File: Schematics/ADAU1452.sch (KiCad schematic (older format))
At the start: 97 parts, among them CN201 COAX, P201 CONN_2x1, P202 CONN_6X2, P203 CONN_6x1, SW201 SWITCH, U201 ADAU1452WBCPZ, U202 ADM13307-5ARZ, U203 25AA1024, X201 24M576

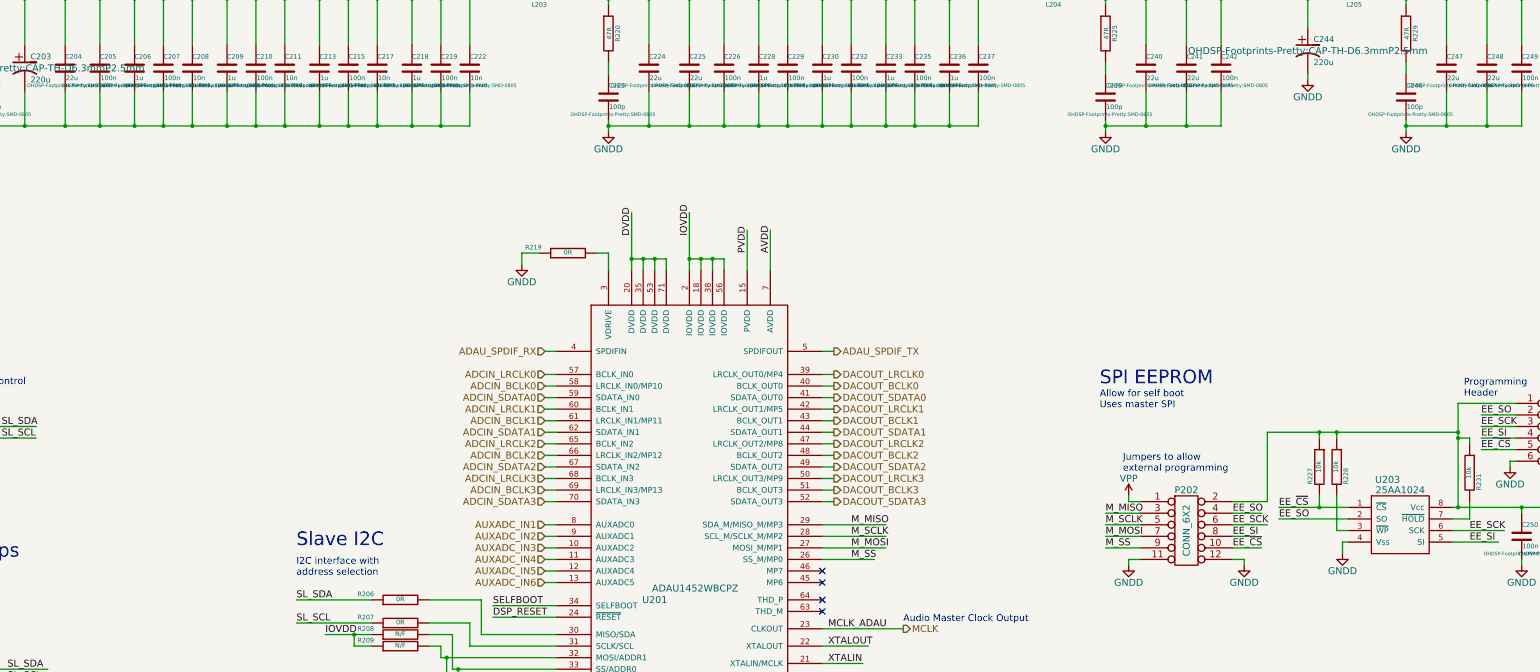
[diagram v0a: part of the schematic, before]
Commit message: WIP
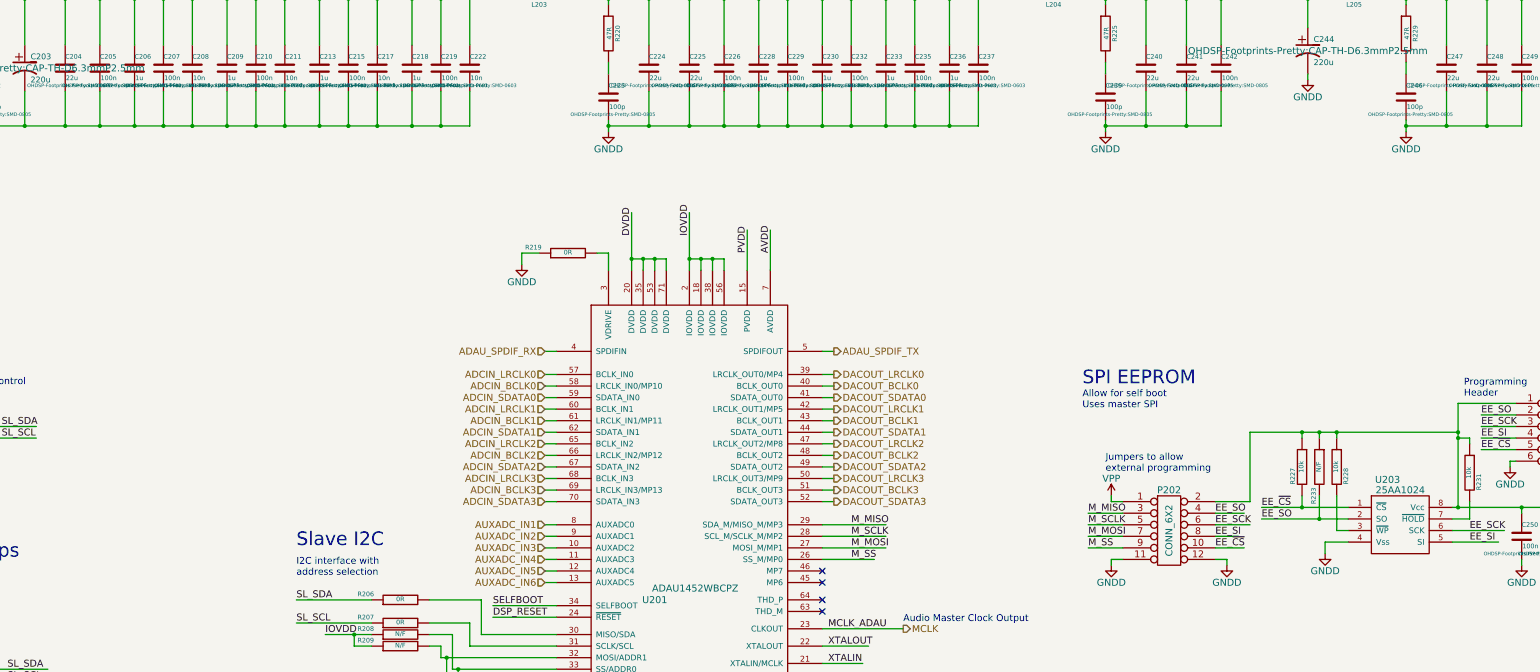
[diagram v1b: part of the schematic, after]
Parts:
- added R233: N/F, OHDSP-Footprints-Pretty:SMD-0805, symbol R
- C206, C207, C208, C209, C210, C211, C213, C215, C217, C218, C219, C222, C228, C229, C230, C232, C233, C235, C236, C237: footprint OHDSP-Footprints-Pretty:SMD-0805 -> OHDSP-Footprints-Pretty:SMD-0603
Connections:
- wire segments 319 -> 321
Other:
- moved on the sheet: P202, R227

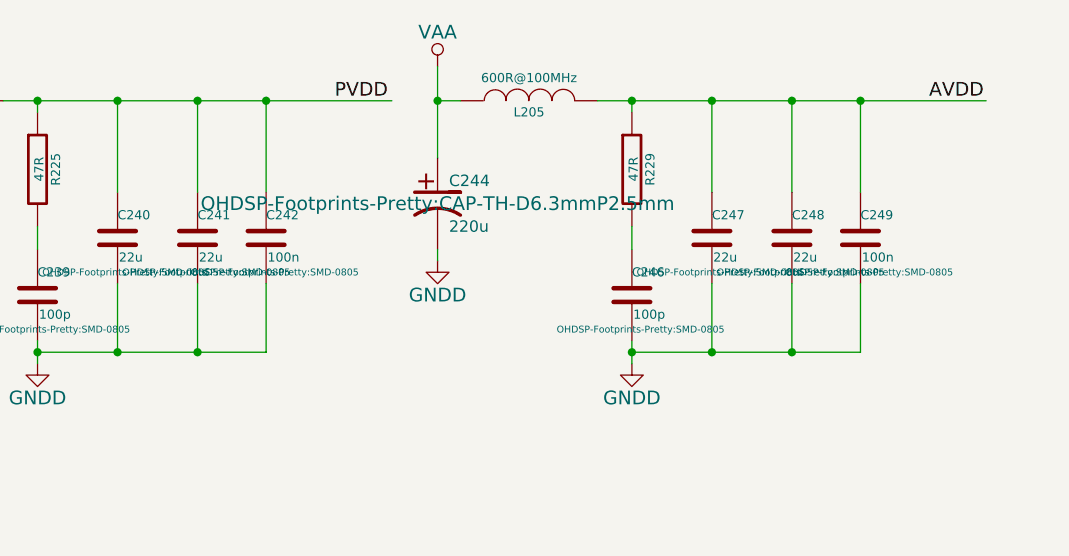
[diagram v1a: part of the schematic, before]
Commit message: WIP
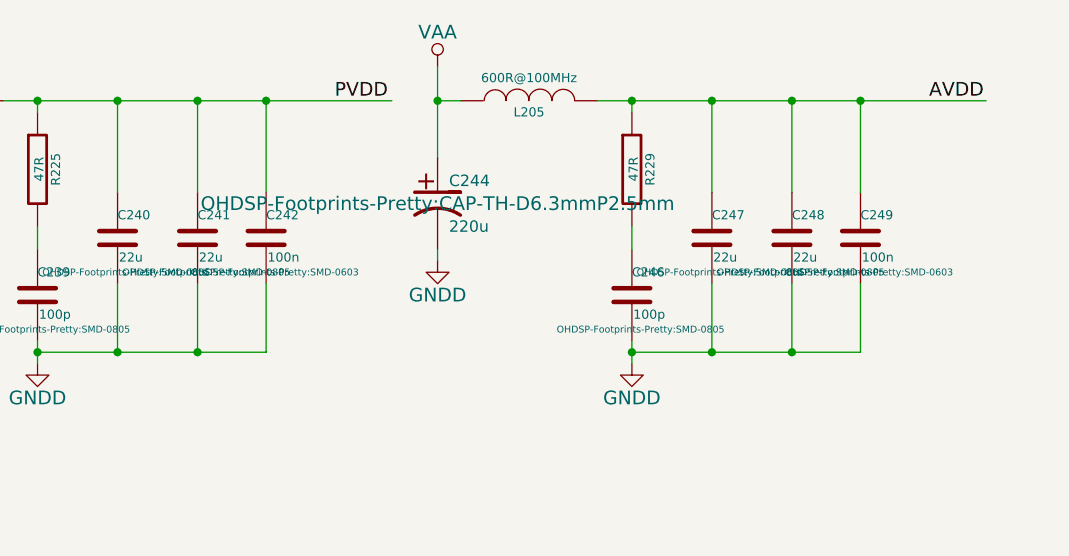
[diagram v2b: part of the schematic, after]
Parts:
- C242, C249: footprint OHDSP-Footprints-Pretty:SMD-0805 -> OHDSP-Footprints-Pretty:SMD-0603
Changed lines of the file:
@@
 F 0 "C242" H 12500 1750 40  0000 L CNN
 F 1 "100n" H 12506 1565 40  0000 L CNN
-F 2 "OHDSP-Footprints-Pretty:SMD-0805" H 12538 1500 30  0000 C CNN
+F 2 "OHDSP-Footprints-Pretty:SMD-0603" H 12538 1500 30  0000 C CNN
 F 3 "~" H 12500 1650 60  0000 C CNN
 	1    12500 1650
@@
 F 0 "C249" H 15100 1750 40  0000 L CNN
 F 1 "100n" H 15106 1565 40  0000 L CNN
-F 2 "OHDSP-Footprints-Pretty:SMD-0805" H 15138 1500 30  0000 C CNN
+F 2 "OHDSP-Footprints-Pretty:SMD-0603" H 15138 1500 30  0000 C CNN
 F 3 "~" H 15100 1650 60  0000 C CNN
 	1    15100 1650
